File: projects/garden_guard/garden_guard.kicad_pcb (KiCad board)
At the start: 4 copper layers, 117 parts, among them IC1 ACPL-227-50CE, IC2 INA226AQDGSRQ1, IC3 INA226AQDGSRQ1, J10 Conn_02x01, J11 Conn_02x01, J12 Mini HDMI, J2 BM04B-SRSS-TB, J3 BM04B-SRSS-TB, J4 Micro_SD_Card_Det, J5 Conn_01x22_Female, J6 Conn_01x22_Female, J7 USB_C_Receptacle_USB2.0, U1 SN74LVC1G07DBVR, U10 TPS2121RUXR, U11 MAX20408AFOF, U12 DMN2028USS-13, U13 DMN2028USS-13, U14 RT9742SNGV, U2 TPD4EUSB30, U3 TPD4EUSB30, U4 RT9742GGJ5, U5 MagJack-A70-112-331N126, U6 AP3441SHE-7B, U7 M.2 Socket, U8 ASEK-32.768KHZ-L-R-T, U9 Ag5810

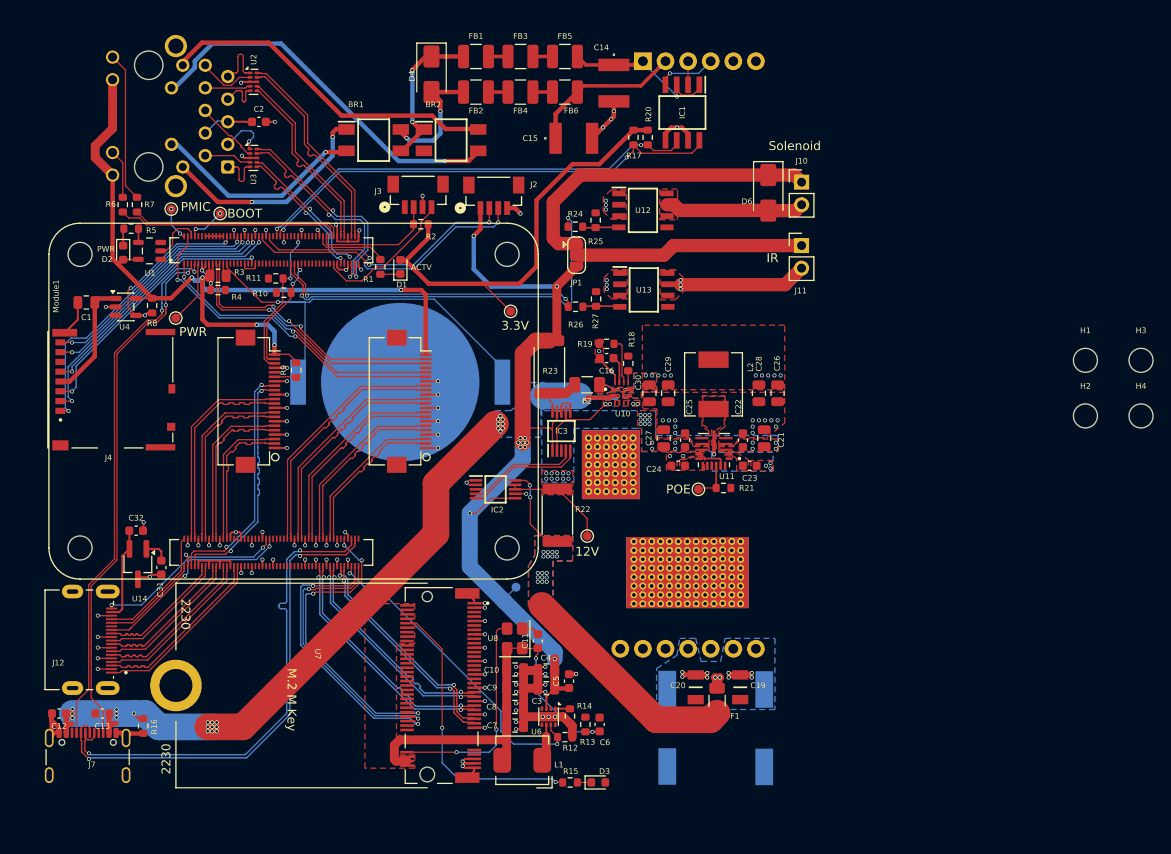
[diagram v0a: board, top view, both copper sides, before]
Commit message: - Still working through DRC - Minor board setup tweaks
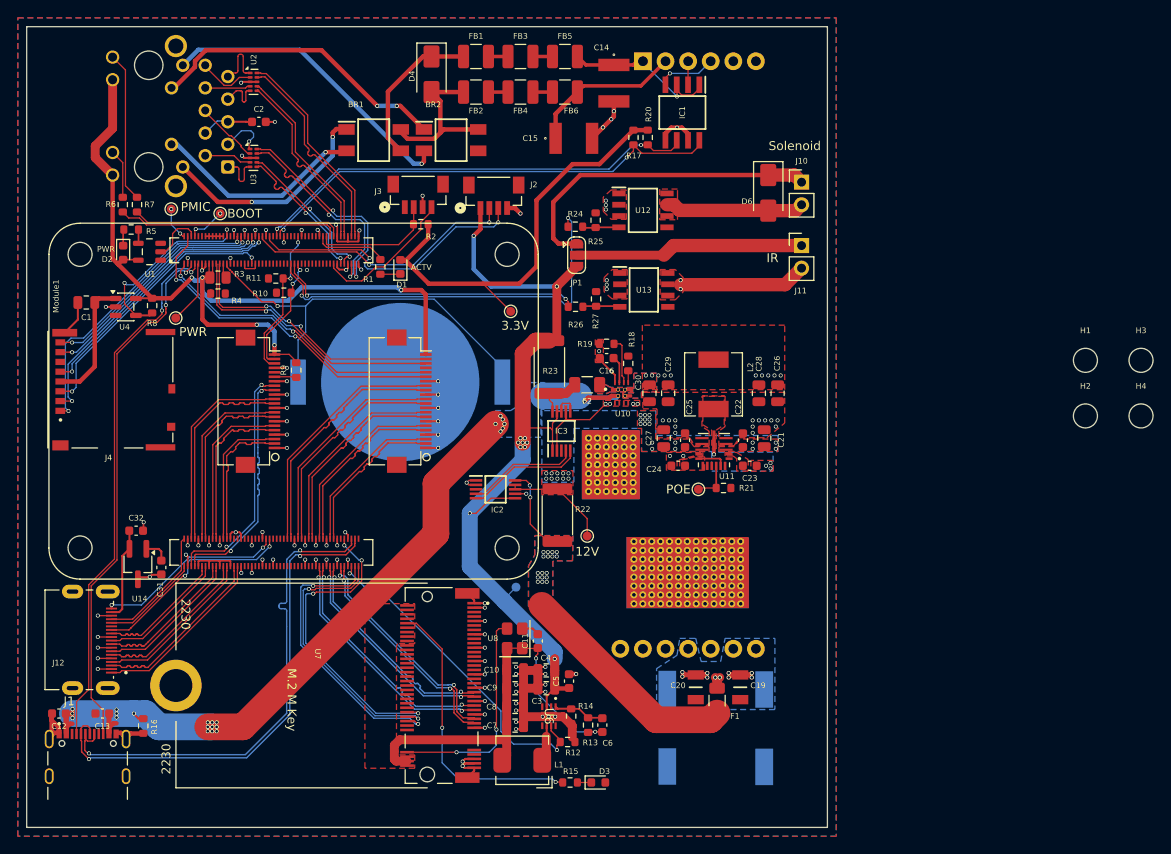
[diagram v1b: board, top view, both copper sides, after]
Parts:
- removed J7: USB_C_Receptacle_USB2.0, Connector_USB:USB_C_Receptacle_GCT_USB4105-xx-A_16P_TopMnt_Horizontal
- added J1: SAMESKY_UJ20-C-H-G-SMT-1-P16-TR, Custom_Connector:UJ20-C-H-G-SMT-1-P16-TR, F.Cu at (58.9, 129.8)
- U6: footprint Package_DFN_QFN:DFN-8-1EP_2x2mm_P0.5mm_EP1.05x1.75mm -> Custom_DCDC:AP3441SHE-7B
- moved R12 0.62 mm to (112.8, 123.4)
- moved R4 0.40 mm to (73.5, 73.0)
- moved C6 0.31 mm to (116.7, 121.5)
- moved R13 0.31 mm to (115.1, 121.5)
- moved R3 0.20 mm to (73.5, 71.2)
- moved R14 0.14 mm to (113.2, 120.5)
- moved U1 0.10 mm to (65.8, 68.3)
- moved R5 0.10 mm to (63.7, 65.8)
- moved U6 0.07 mm to (110.7, 120.5)
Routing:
- net /CM5_HighSpeed/TR2_TAP: track 42.9 -> 34.2 mm, vias 1 -> 2
- net Net-(BR1--): track 14.2 -> 18.4 mm, vias 2 -> 0
- net /CM5_HighSpeed/TR3_TAP: track 38.5 -> 34.4 mm, vias 0 -> 1
- net /PCIe-M2/FB: track 1.66 -> 5.65 mm
- net /CM5_HighSpeed/+1.8v: track 4.33 -> 1.74 mm, vias 2 -> 1
- net /+3.3v: track 145.4 -> 147.5 mm
- net /CM5_HighSpeed/SD_PWR_ON: track 19.0 -> 21.0 mm, vias 3 -> 2
- net /CM5_HighSpeed/VBAT: track 50.3 -> 48.3 mm
- net GND: track 179.2 -> 180.4 mm, vias 122 -> 125
- net /CM5_GPIO (Ethernet, GPIO, MicroSD)/PCIE_PWR_EN: track 36.1 -> 37.1 mm
- net /CM5_HighSpeed/TRD0_N: track 21.8 -> 22.6 mm
- net /CM5_HighSpeed/SD_PWR: track 13.6 -> 14.3 mm
- net /CM5_HighSpeed/SD_CMD: track 29.9 -> 30.5 mm
- net /CM5_HighSpeed/UART0_TX: track 31.3 -> 30.7 mm
- net Net-(BR1-+): track 17.6 -> 17.4 mm, vias 2 -> 0
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- added copper zone on B.Cu, net GND
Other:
- board outline added: 90 x 90 mm
